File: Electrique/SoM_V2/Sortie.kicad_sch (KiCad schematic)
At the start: 8 parts, among them U401 PCA9633DP1

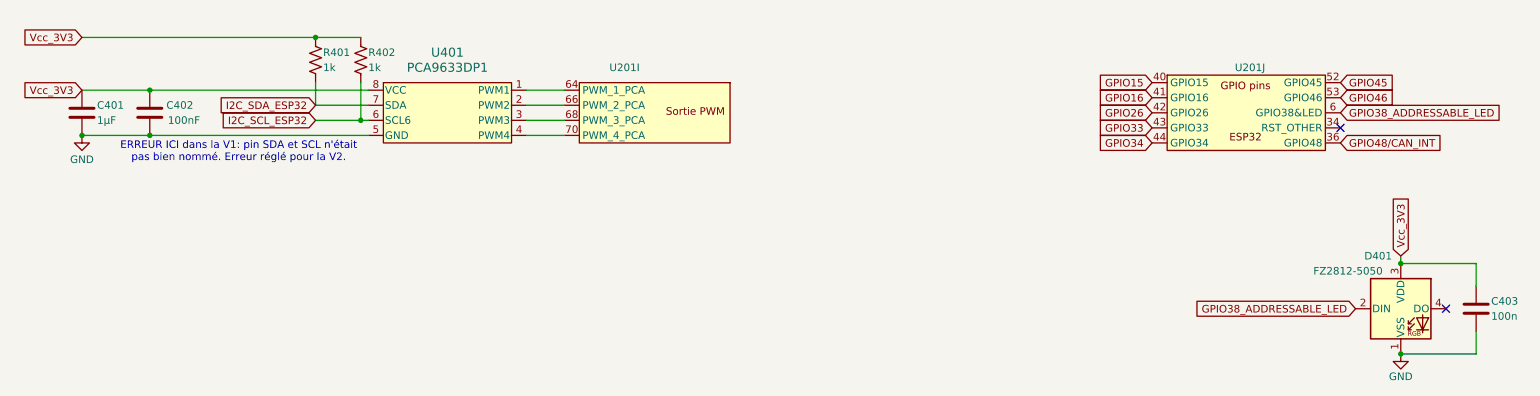
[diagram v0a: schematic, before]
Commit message: Clean up schema et PCB
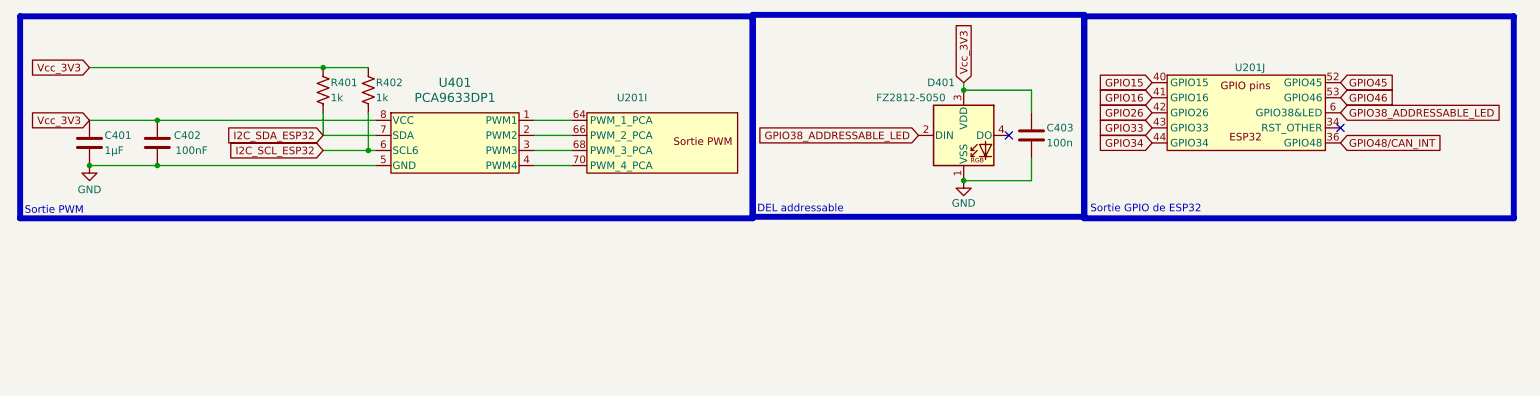
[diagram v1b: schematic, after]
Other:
- note added: "DEL addressable"
- note added: "Sortie GPIO de ESP32"
- note added: "Sortie PWM"
- note removed: "ERREUR ICI dans la V1: pin SDA et SCL n'était pas bien nommé. Erreur réglé pour la V2."
- moved on the sheet: C401, C402, C403, D401, R401, R402, U201I, U401
